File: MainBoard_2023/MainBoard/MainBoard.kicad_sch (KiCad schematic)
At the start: 27 parts

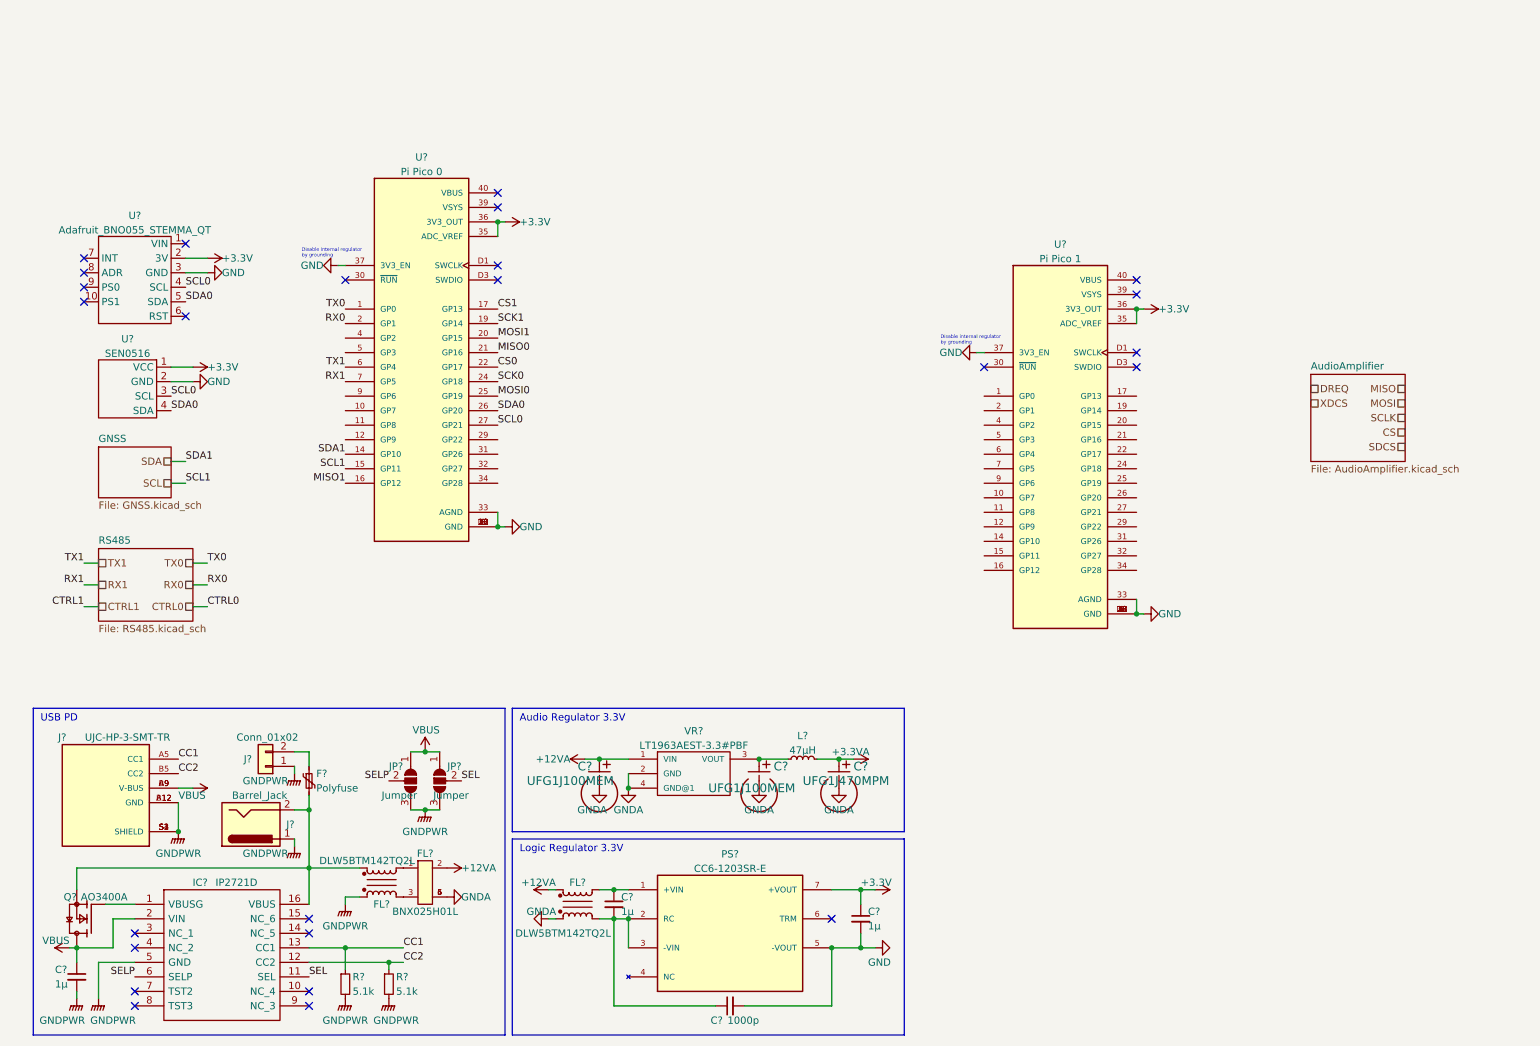
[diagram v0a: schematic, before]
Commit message: pico*2の場合
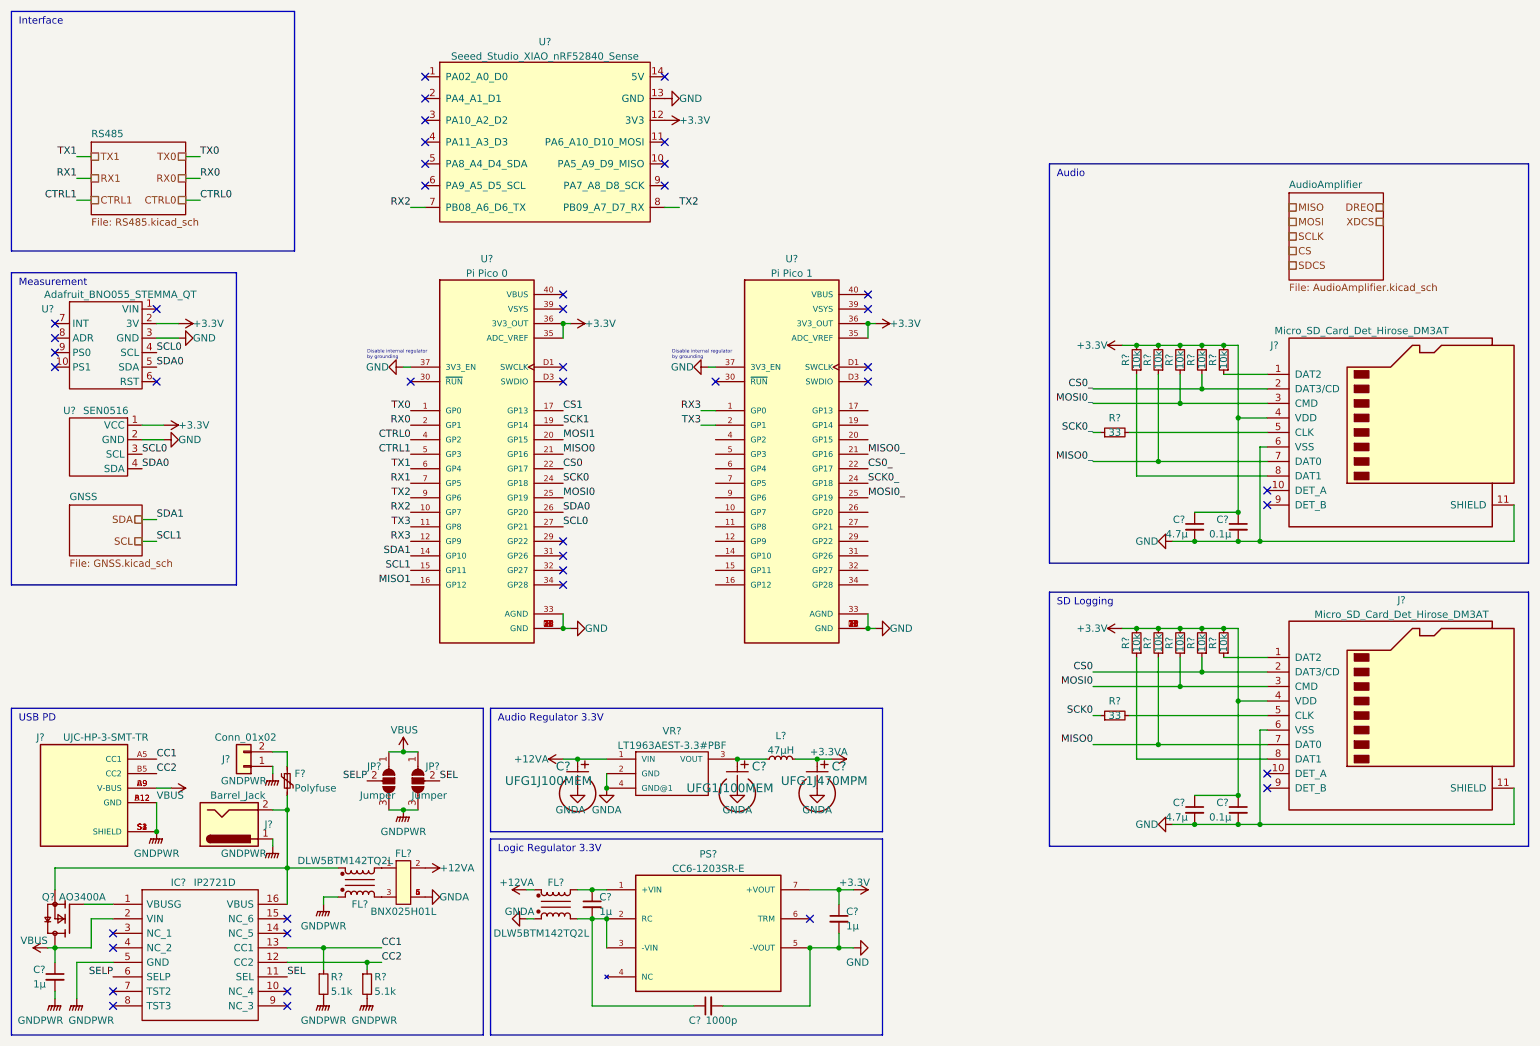
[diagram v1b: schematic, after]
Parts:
- added C? (x2): 4.7μ, symbol Device:C_Small
- added C? (x2): 0.1μ, symbol Device:C_Small
- added J? (x2): Micro_SD_Card_Det_Hirose_DM3AT, symbol Connector:Micro_SD_Card_Det_Hirose_DM3AT
- added R? (x10): 10k, symbol Device:R_Small
- added R? (x2): 33, symbol Device:R_Small
- added U?: Seeed_Studio_XIAO_nRF52840_Sense, symbol Seeed_Studio_XIAO_nRF52840_Sense:Seeed_Studio_XIAO_nRF52840_Sense
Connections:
- net +3.3V: now also C?.1, C?.1, C?.1, C?.1, J?.4 (VDD), J?.4 (VDD), R?.2, R?.2, R?.2, R?.2, R?.2, R?.2, R?.2, R?.2, R?.2, R?.2, U?.12 (3V3)
- net CS0: now also J?.2 (DAT3/CD), R?.1
- net CTRL0: now also U?.4 (GP2)
- net CTRL1: now also U?.5 (GP3)
- net GND: now also C?.2, C?.2, C?.2, C?.2, J?.11 (SHIELD), J?.11 (SHIELD), J?.6 (VSS), J?.6 (VSS), U?.13 (GND)
- net MISO0: now also J?.7 (DAT0), R?.1
- net MOSI0: now also J?.3 (CMD), R?.1
- net SCK0: now also R?.1
- net RX2: now reaches U?.10 (GP7)
- net RX2: now also U?.7 (PB08_A6_D6_TX)
- net TX3: now reaches U?.11 (GP8)
- net TX3: now also U?.2 (GP1)
- net RX3: now reaches U?.12 (GP9)
- net RX3: now also U?.1 (GP0)
- net TX2: now reaches U?.9 (GP6)
- net TX2: now also U?.8 (PB09_A7_D7_RX)
- net MISO0_: now reaches U?.21 (GP16)
- net MISO0_: now also J?.7 (DAT0), R?.1
- net CS0_: now reaches U?.22 (GP17)
- net CS0_: now also J?.2 (DAT3/CD), R?.1
- net SCK0_: now reaches U?.24 (GP18)
- net SCK0_: now also R?.1
- net MOSI0_: now reaches U?.25 (GP19)
- net MOSI0_: now also J?.3 (CMD), R?.1
- new net: J?.8 (DAT1), R?.1 (x2)
- new net: J?.5 (CLK), R?.2 (x2)
- new net: J?.1 (DAT2), R?.1 (x2)
- no-connect marks 25 -> 43
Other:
- note added: "Audio"
- note added: "Interface"
- note added: "Measurement"
- note added: "SD Logging"
- moved on the sheet: C?, F?, FL?, IC?, J?, JP?, L?, PS?, Q?, R?, U?, VR?
